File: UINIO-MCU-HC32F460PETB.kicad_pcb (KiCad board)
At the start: 2 copper layers, 93.7 x 53.1 mm, 55 parts, among them J1 Conn_01x18_Pin, J2 Conn_01x34_Pin, J3 Conn_01x34_Pin, J4 MD, J5 Conn_01x04_Pin, J6 Conn_01x04_Pin, J7 Conn_01x04_Pin, J8 Conn_01x04_Pin, J9 Conn_01x04_Pin, SW1 NRST, U1 ME6211C33M5G, U2 HC32F460PETB-LQFP100, Y1 32.768KHz, Y2 8MHz

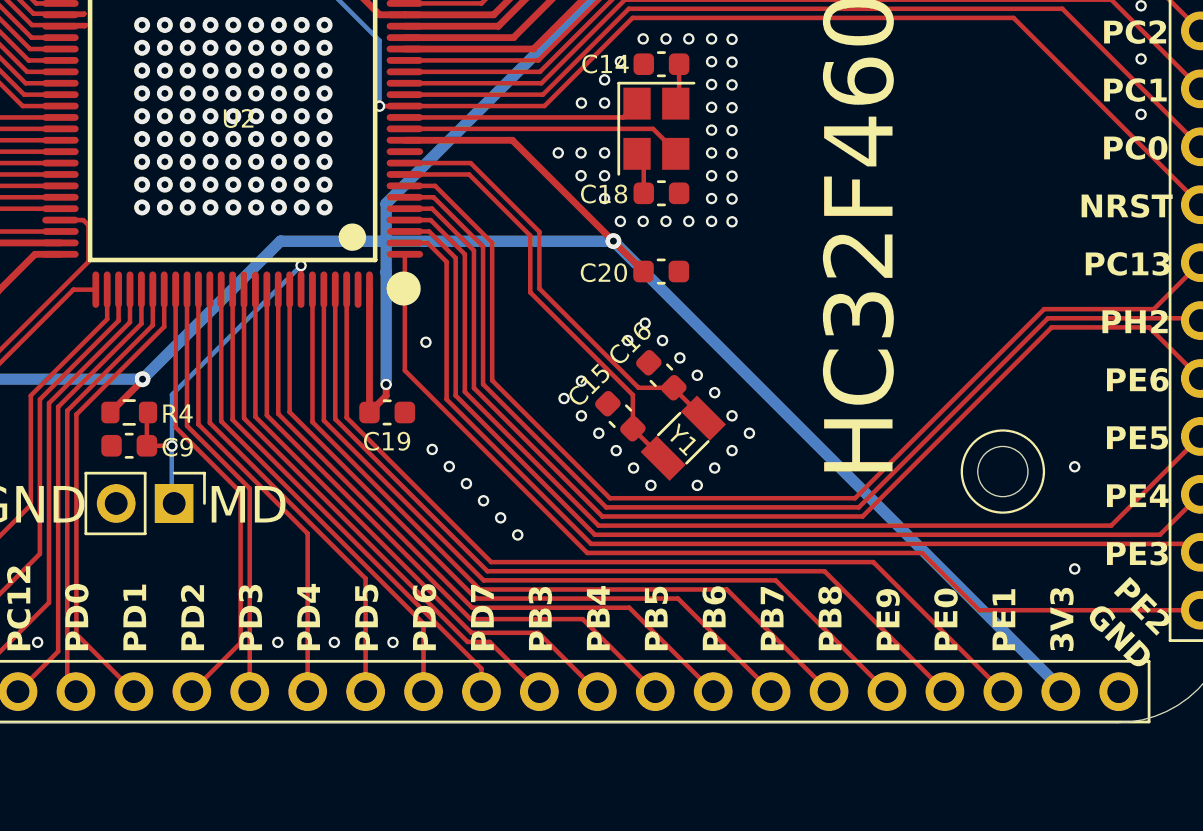
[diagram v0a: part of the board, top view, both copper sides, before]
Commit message: update
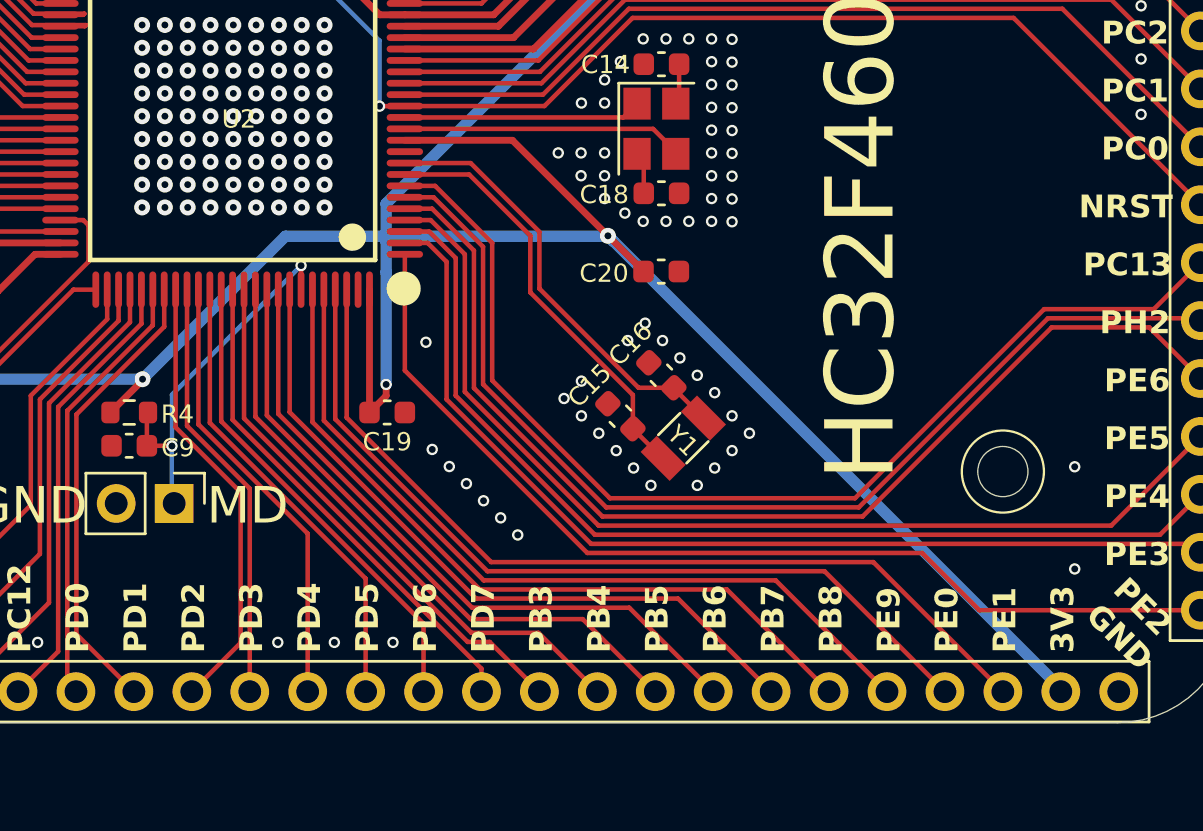
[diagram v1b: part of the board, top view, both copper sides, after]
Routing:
- net VCC_3.3V: track 331.5 -> 332.8 mm
